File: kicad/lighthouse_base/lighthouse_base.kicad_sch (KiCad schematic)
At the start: 8 parts, among them J1 USB_C_Receptacle_USB2.0_14P, J2 Barrel_Jack_Switch

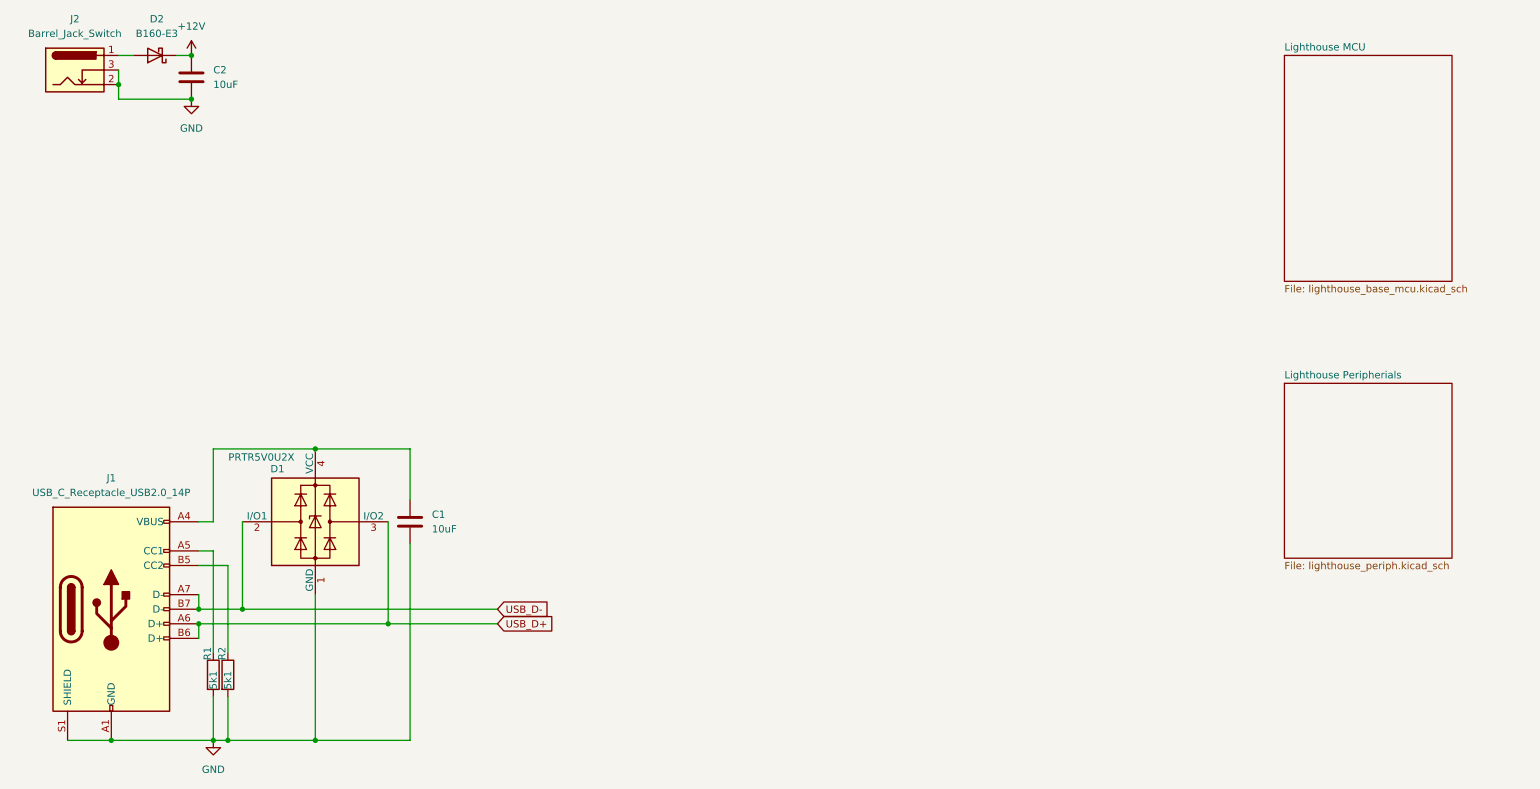
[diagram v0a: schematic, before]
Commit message: schema v1 done
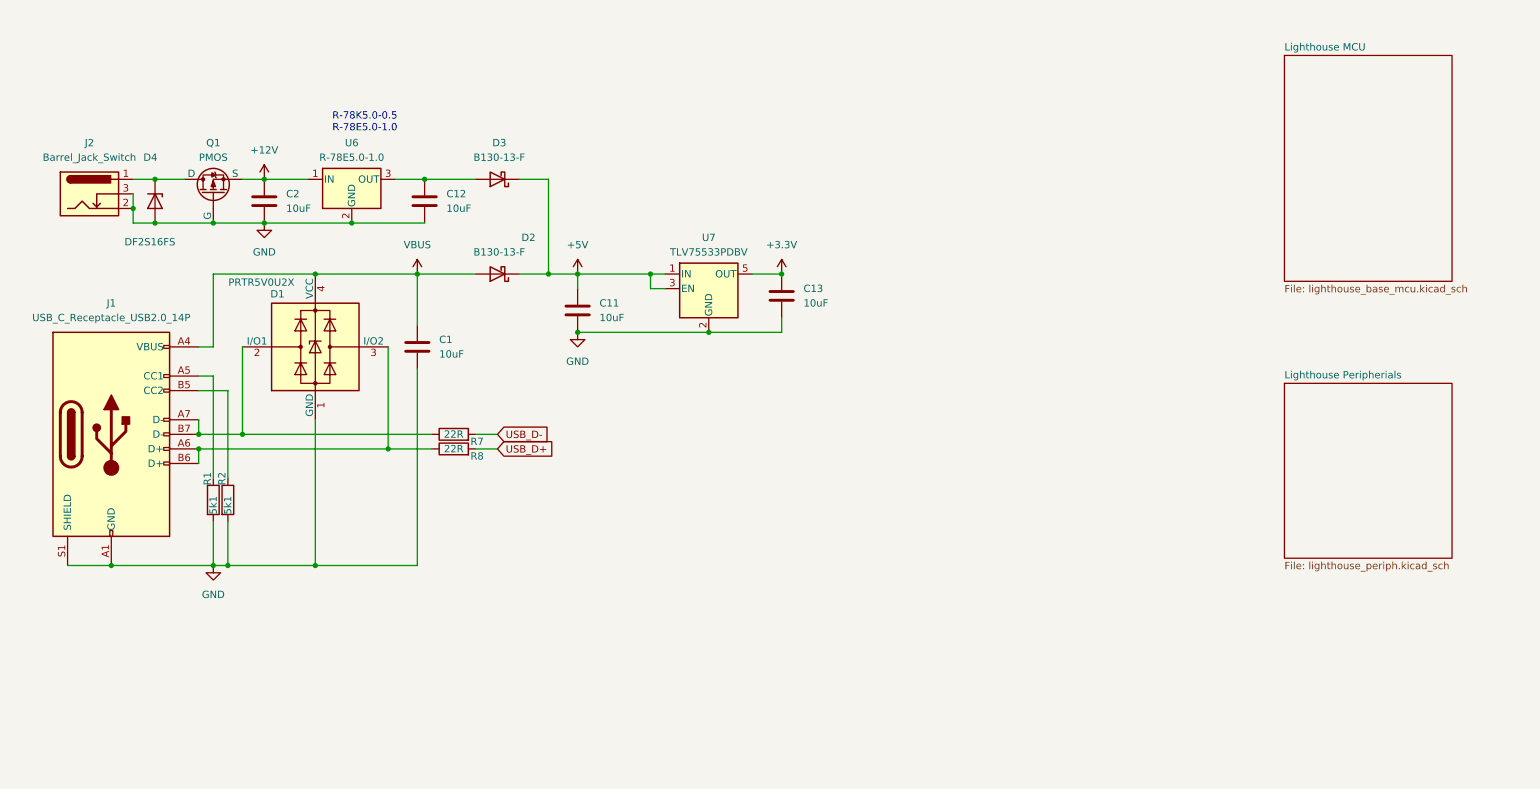
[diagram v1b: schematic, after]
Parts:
- removed D2: B160-E3, Diode_SMD:D_SMA, symbol Diode:B160-E3
- added C11, C12, C13: 10uF, symbol Device:C
- added D2, D3: B130-13-F, symbol Device:D_Schottky
- added D4: DF2S16FS, Diode_SMD:D_SOD-523, symbol Diode:ESD5Zxx
- added Q1: PMOS, symbol Simulation_SPICE:PMOS
- added R7, R8: 22R, symbol Device:R
- added U6: R-78E5.0-1.0, Converter_DCDC:Converter_DCDC_RECOM_R-78E-0.5_THT, symbol Regulator_Switching:R-78E5.0-1.0
- added U7: TLV75533PDBV, Package_TO_SOT_SMD:SOT-23-5, symbol Regulator_Linear:TLV75533PDBV
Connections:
- net +12V: now also Q1.3 (S), U6.1 (IN)
- net GND: now also C11.2, C12.2, C13.2, D4.2 (A), Q1.2 (G), U6.2 (GND), U7.2 (GND)
- net USB_D+: now also R8.2; no longer D1.3 (I/O2), J1.A6 (D+), J1.B6 (D+)
- net USB_D-: now also R7.2; no longer D1.2 (I/O1), J1.A7 (D-), J1.B7 (D-)
- net VBUS: now reaches C1.1, D1.4 (VCC), J1.A4 (VBUS), J1.A9 (VBUS), J1.B4 (VBUS), J1.B9 (VBUS)
- net VBUS: now also D2.2 (A)
- net at J2.1: now also D4.1 (K), Q1.1 (D)
- new net: D1.3 (I/O2), J1.A6 (D+), J1.B6 (D+), R8.1
- new net: D1.2 (I/O1), J1.A7 (D-), J1.B7 (D-), R7.1
- new net: C12.1, D3.2 (A), U6.3 (OUT)
- new net +3.3V: C13.1, U7.5 (OUT)
- new net +5V: C11.1, D2.1 (K), D3.1 (K), U7.1 (IN), U7.3 (EN)
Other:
- note added: "R-78K5.0-0.5 R-78E5.0-1.0"
- moved on the sheet: C1, C2, D1, J1, J2, R1, R2

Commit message: schematics done
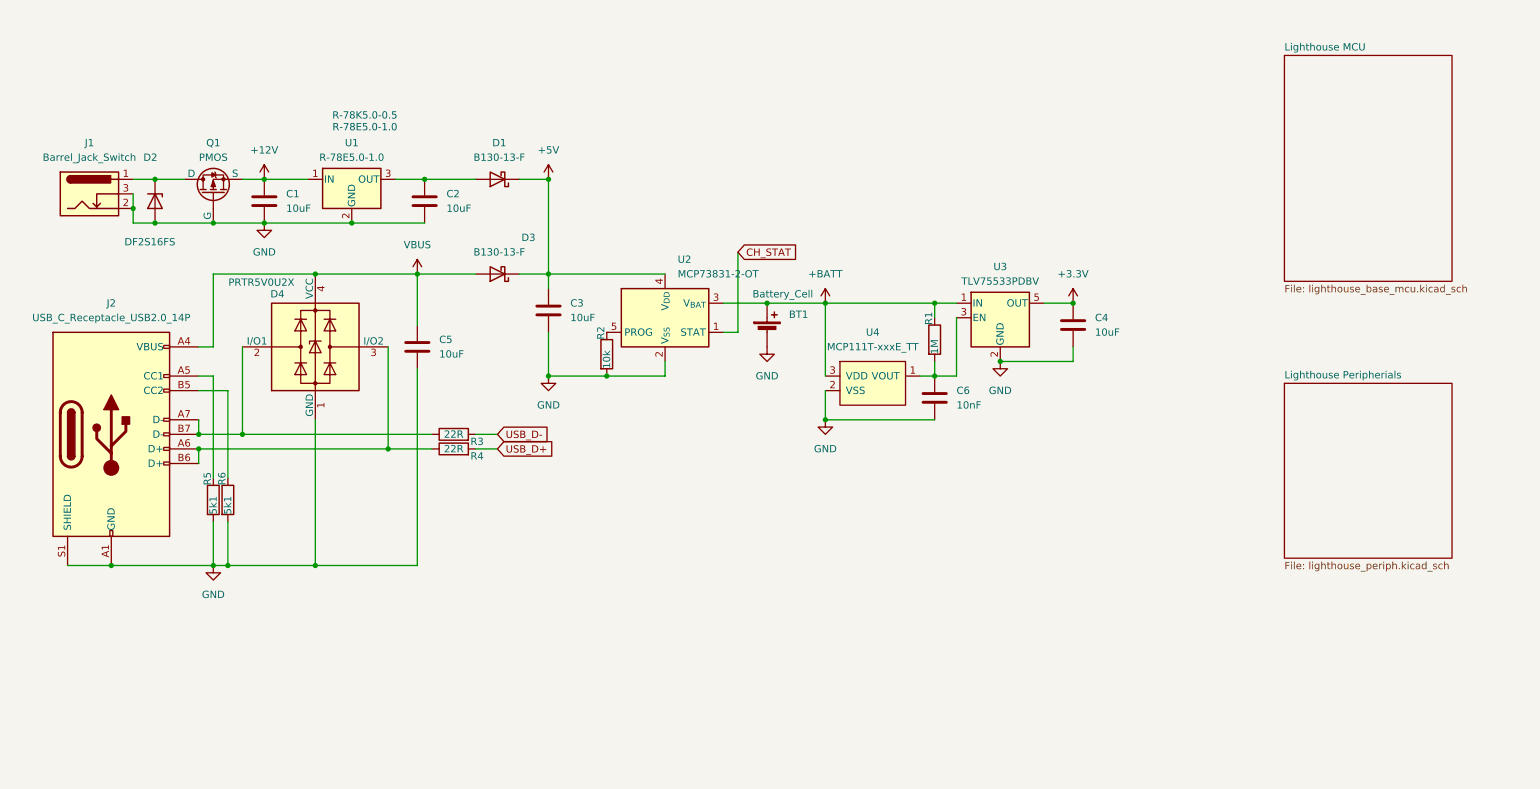
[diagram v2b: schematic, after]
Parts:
- added BT1: Battery_Cell, Connector_PinHeader_2.54mm:PinHeader_1x02_P2.54mm_Vertical, symbol Device:Battery_Cell
- added C6: 10nF, Capacitor_SMD:C_0201_0603Metric_Pad0.64x0.40mm_HandSolder, symbol Device:C
- added R1: 1M, Resistor_SMD:R_0603_1608Metric_Pad0.98x0.95mm_HandSolder, symbol Device:R
- added R2: 10k, Resistor_SMD:R_0603_1608Metric_Pad0.98x0.95mm_HandSolder, symbol Device:R
- added U2: MCP73831-2-OT, Package_TO_SOT_SMD:SOT-23-5, symbol Battery_Management:MCP73831-2-OT
- added U4: MCP111T-xxxE_TT, Package_TO_SOT_SMD:SOT-23-3, symbol MEgliParts:MCP111T-xxxE_TT
- C1: renamed from C2; footprint (none) -> Capacitor_SMD:C_0805_2012Metric_Pad1.18x1.45mm_HandSolder
- C2: renamed from C12; footprint (none) -> Capacitor_SMD:C_0805_2012Metric_Pad1.18x1.45mm_HandSolder
- C3: renamed from C11; footprint (none) -> Capacitor_SMD:C_0805_2012Metric_Pad1.18x1.45mm_HandSolder
- C4: renamed from C13; footprint (none) -> Capacitor_SMD:C_0805_2012Metric_Pad1.18x1.45mm_HandSolder
- C5: renamed from C1; footprint (none) -> Capacitor_SMD:C_0805_2012Metric_Pad1.18x1.45mm_HandSolder
- D1: renamed from D3; footprint (none) -> Diode_SMD:D_SMA_Handsoldering
- D3: renamed from D2; footprint (none) -> Diode_SMD:D_SMA_Handsoldering
- Q1: footprint (none) -> Package_TO_SOT_SMD:SOT-23
- R3: renamed from R7; footprint (none) -> Resistor_SMD:R_0603_1608Metric_Pad0.98x0.95mm_HandSolder
- R4: renamed from R8; footprint (none) -> Resistor_SMD:R_0603_1608Metric_Pad0.98x0.95mm_HandSolder
- R5: renamed from R1; footprint (none) -> Resistor_SMD:R_0603_1608Metric_Pad0.98x0.95mm_HandSolder
- R6: renamed from R2; footprint (none) -> Resistor_SMD:R_0603_1608Metric_Pad0.98x0.95mm_HandSolder
- renumbered D4 to D2, D1 to D4, J2 to J1, J1 to J2, U6 to U1, U7 to U3
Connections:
- net +5V: now also U2.4 (V_{DD}); no longer U3.1 (IN), U3.3 (EN)
- net GND: now also BT1.2 (-), C6.2, R2.2, U2.2 (V_{SS}), U4.2 (VSS)
- new net: C6.1, R1.2, U3.3 (EN), U4.1 (VOUT)
- new net: R2.1, U2.5 (PROG)
- new net +BATT: BT1.1 (+), R1.1, U2.3 (V_{BAT}), U3.1 (IN), U4.3 (VDD)
- new net CH_STAT: U2.1 (STAT)
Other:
- moved on the sheet: C3, C4, U3
